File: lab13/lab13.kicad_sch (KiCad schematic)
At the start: 16 parts, among them U1 74LS73, U2 74LS73, U3 74LS73, U4 74LS73, U5 74LS08, U6 74LS08

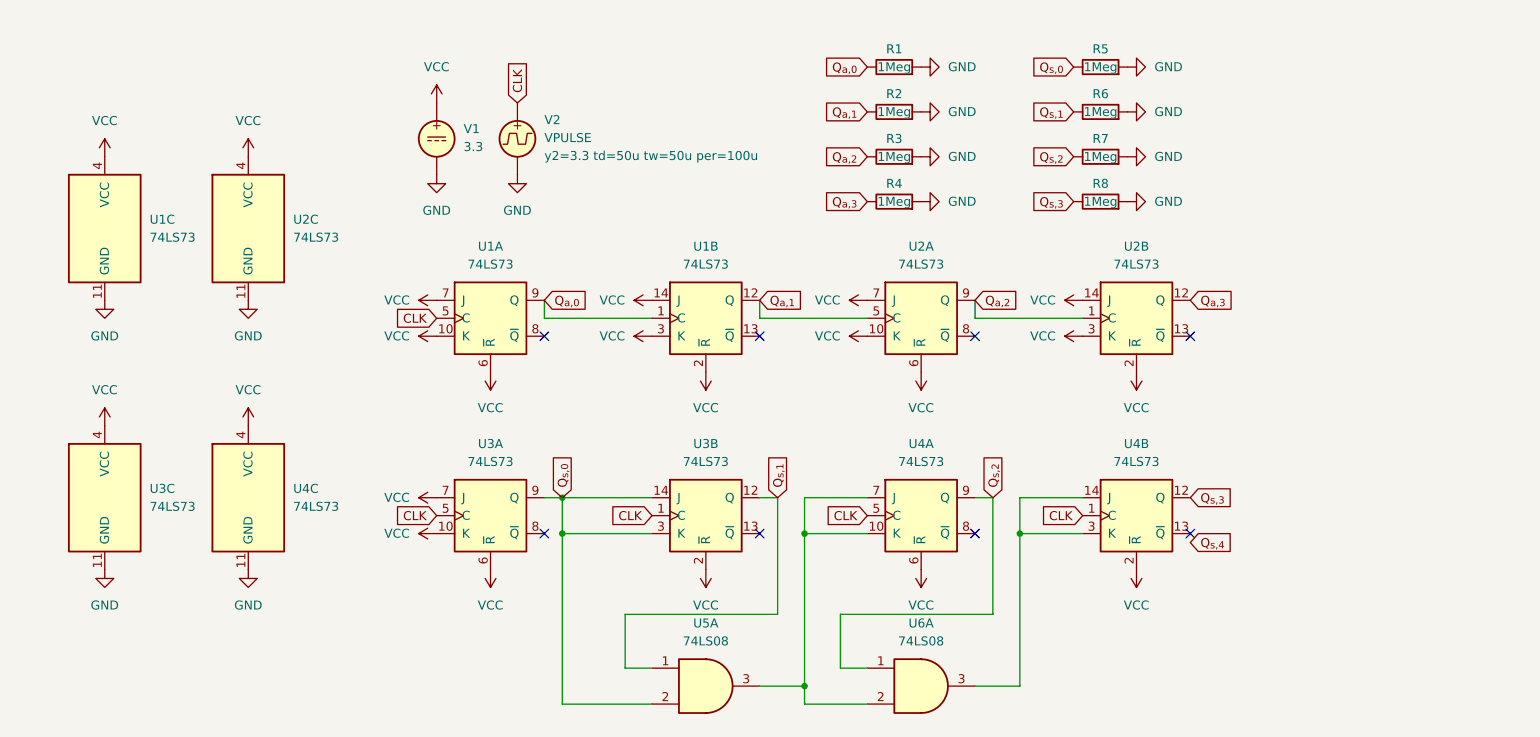
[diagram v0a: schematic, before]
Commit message: update lab13
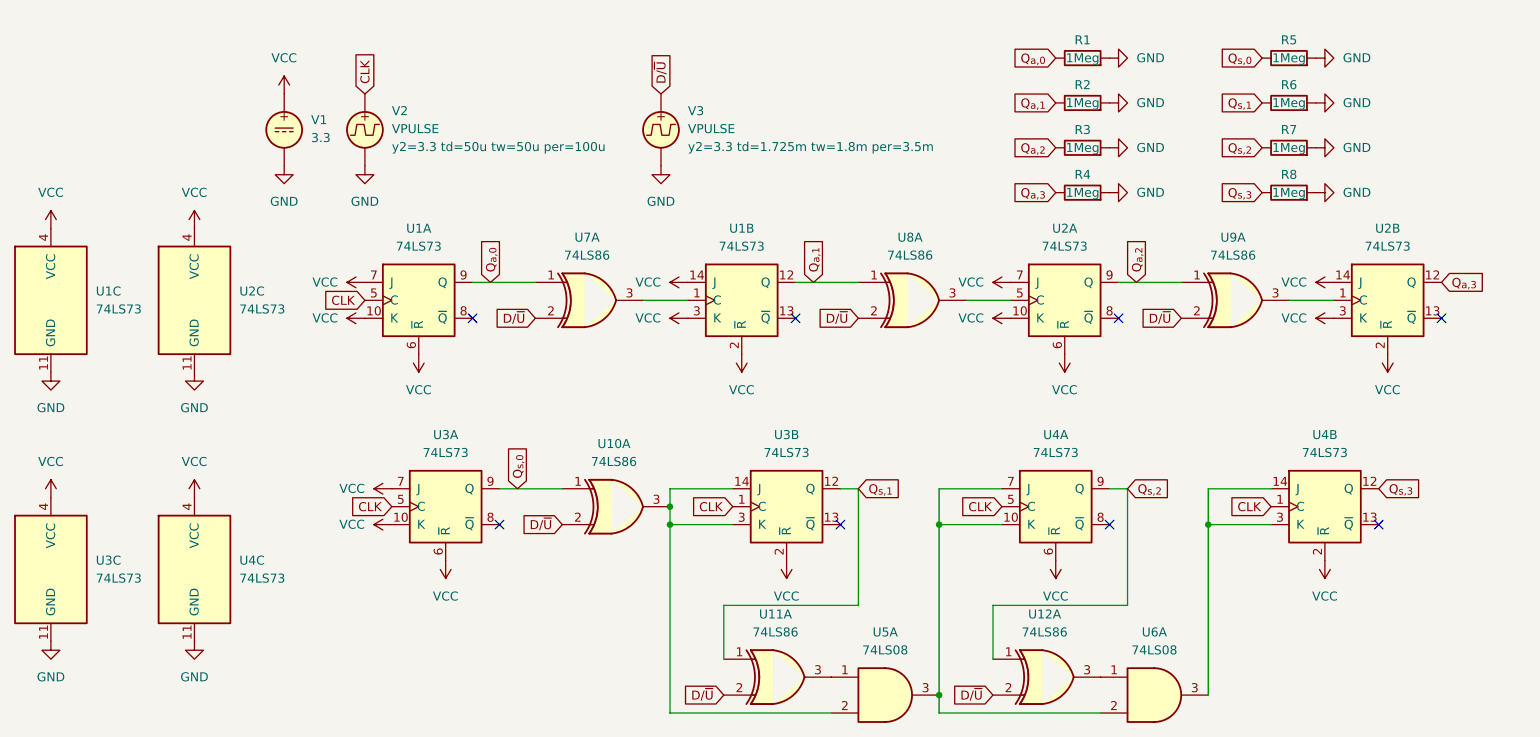
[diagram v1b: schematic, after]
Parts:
- added U10, U11, U12, U7, U8, U9: 74LS86, symbol 74xx:74LS86
- added V3: VPULSE, symbol Simulation_SPICE:VPULSE
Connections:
- net GND: now also V3.2
- net Q_{a,0}: now also U7.1; no longer U1.1 (C)
- net Q_{a,1}: now also U8.1; no longer U2.5 (C)
- net Q_{a,2}: now also U9.1; no longer U2.1 (C)
- net Q_{s,0}: now also U10.1; no longer U3.14 (J), U3.3 (K), U5.2
- net Q_{s,1}: now also U11.1; no longer U5.1
- net Q_{s,2}: now also U12.1; no longer U6.1
- new net: U1.1 (C), U7.3
- new net: U11.3, U5.1
- new net: U10.3, U3.14 (J), U3.3 (K), U5.2
- new net: U2.5 (C), U8.3
- new net: U2.1 (C), U9.3
- new net: U12.3, U6.1
- new net D/~{U}: U10.2, U11.2, U12.2, U7.2, U8.2, U9.2, V3.1
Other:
- moved on the sheet: R1, R2, R3, R4, R5, R6, R7, R8, U1A, U1B, U1C, U2A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
